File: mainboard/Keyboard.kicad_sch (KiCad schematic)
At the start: 111 parts, among them J10 Joystick, J11 Keyboard, J9 Cassette, Q3 TIS92, Q4 TIS92, Q5 TIS92, Q6 TIS92, Q7 TIS92, Q8 TIS92, Q9 TIS92, U21 RC4558, U36 TMS9901, U37 74LS156, U38 TIL119, U39 TIL119

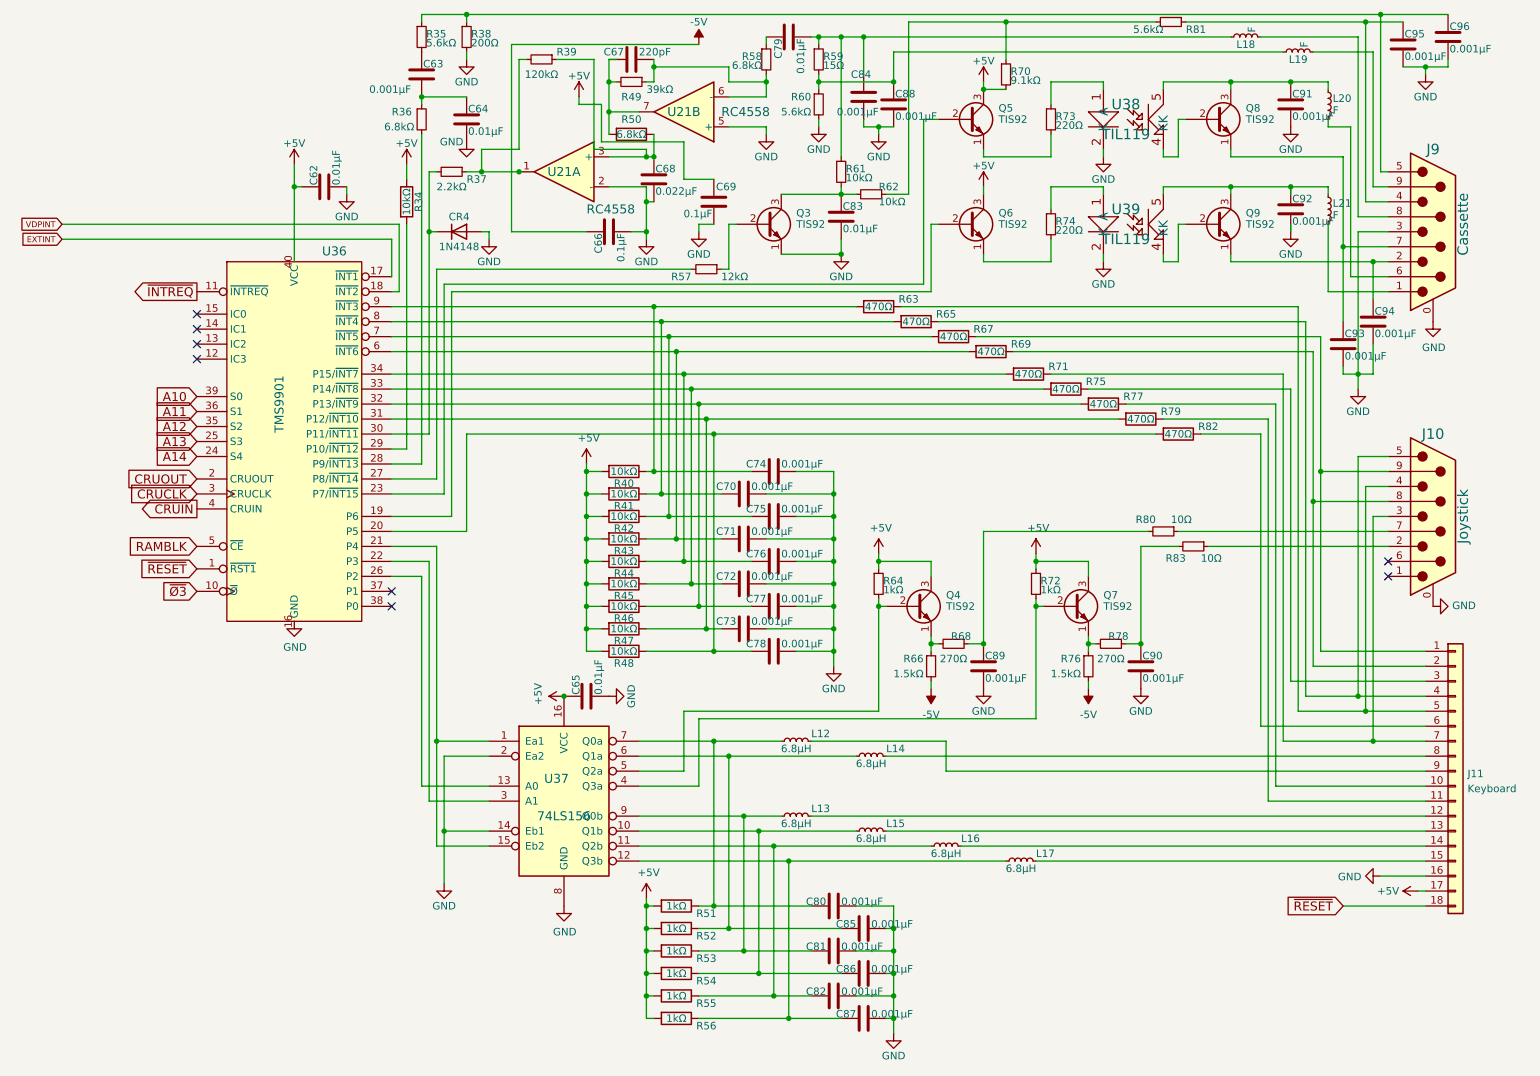
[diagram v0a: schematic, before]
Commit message: PCB rework
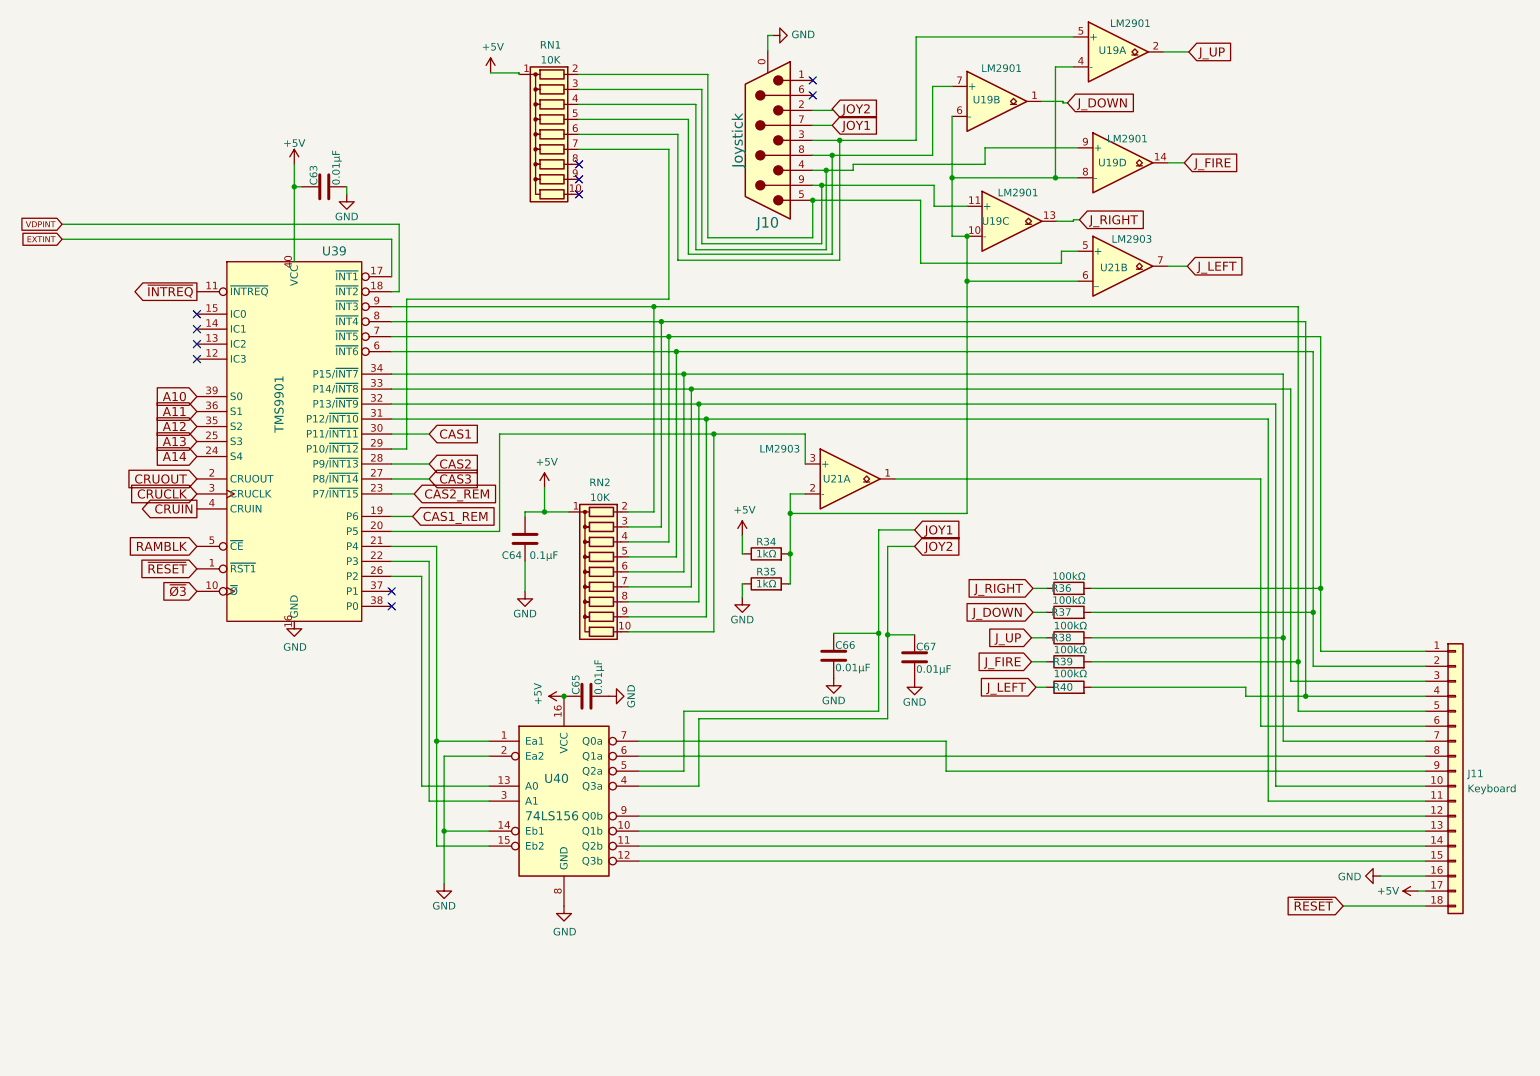
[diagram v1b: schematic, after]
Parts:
- removed C63, C70, C71, C72, C73, C75, C76, C77, C78, C80, C81, C82, C84, C85, C86, C87, C88, C91, C92, C93, C94, C95, C96: 0.001µF, Capacitor_THT:C_Rect_L7.0mm_W2.0mm_P5.00mm, symbol Device:C
- removed C64, C79, C83: 0.01µF, Capacitor_THT:C_Rect_L7.0mm_W2.0mm_P5.00mm, symbol Device:C
- removed C66, C69: 0.1µF, Capacitor_THT:C_Rect_L7.0mm_W2.0mm_P5.00mm, symbol Device:C
- removed C67: 220pF, Capacitor_THT:C_Rect_L7.0mm_W2.0mm_P5.00mm, symbol Device:C
- removed C68: 0.022µF, Capacitor_THT:C_Rect_L7.0mm_W2.0mm_P5.00mm, symbol Device:C
- removed CR4: 1N4148, Diode_THT:D_A-405_P7.62mm_Horizontal, symbol Device:D
- removed J9: Cassette, Connector_Dsub:DSUB-9_Female_Horizontal_P2.77x2.84mm_EdgePinOffset4.94mm_Housed_MountingHolesOffset7.48mm, symbol Connector:DB9_Male_MountingHoles
- removed L12, L13, L14, L15, L16, L17: 6.8µH, Resistor_THT:R_Axial_DIN0207_L6.3mm_D2.5mm_P7.62mm_Horizontal, symbol Device:L_Small
- removed L18, L19, L20, L21: F, Resistor_THT:R_Axial_DIN0207_L6.3mm_D2.5mm_P7.62mm_Horizontal, symbol Device:L_Small
- removed Q3, Q4, Q5, Q6, Q7, Q8, Q9: TIS92, Package_TO_SOT_THT:TO-92_HandSolder, symbol Device:Q_NPN_EBC
- removed R35, R60, R81: 5.6kΩ, Resistor_THT:R_Axial_DIN0207_L6.3mm_D2.5mm_P7.62mm_Horizontal, symbol Device:R_Small
- removed R36, R58: 6.8kΩ, Resistor_THT:R_Axial_DIN0207_L6.3mm_D2.5mm_P7.62mm_Horizontal, symbol Device:R_Small
- removed R37: 2.2kΩ, Resistor_THT:R_Axial_DIN0207_L6.3mm_D2.5mm_P7.62mm_Horizontal, symbol Device:R_Small
- removed R38: 200Ω, Resistor_THT:R_Axial_DIN0207_L6.3mm_D2.5mm_P7.62mm_Horizontal, symbol Device:R_Small
- removed R39: 120kΩ, Resistor_THT:R_Axial_DIN0207_L6.3mm_D2.5mm_P7.62mm_Horizontal, symbol Device:R_Small
- removed R41, R42, R43, R44, R45, R46, R47, R48: 10kΩ, Resistor_THT:R_Axial_DIN0207_L6.3mm_D2.5mm_P7.62mm_Horizontal, symbol Device:R
- removed R49: 39kΩ, Resistor_THT:R_Axial_DIN0207_L6.3mm_D2.5mm_P7.62mm_Horizontal, symbol Device:R_Small
- removed R50: 6.8kΩ, Resistor_THT:R_Axial_DIN0207_L6.3mm_D2.5mm_P7.62mm_Horizontal, symbol Device:R
- removed R51, R52, R53, R54, R55, R56: 1kΩ, Resistor_THT:R_Axial_DIN0207_L6.3mm_D2.5mm_P7.62mm_Horizontal, symbol Device:R
- removed R57: 12kΩ, Resistor_THT:R_Axial_DIN0207_L6.3mm_D2.5mm_P7.62mm_Horizontal, symbol Device:R_Small
- removed R59: 15Ω, Resistor_THT:R_Axial_DIN0207_L6.3mm_D2.5mm_P7.62mm_Horizontal, symbol Device:R_Small
- removed R61, R62: 10kΩ, Resistor_THT:R_Axial_DIN0207_L6.3mm_D2.5mm_P7.62mm_Horizontal, symbol Device:R_Small
- removed R63, R65, R67, R69, R71, R75, R77, R79, R82: 470Ω, Resistor_THT:R_Axial_DIN0207_L6.3mm_D2.5mm_P7.62mm_Horizontal, symbol Device:R
- removed R64, R72: 1kΩ, Resistor_THT:R_Axial_DIN0207_L6.3mm_D2.5mm_P7.62mm_Horizontal, symbol Device:R_Small
- removed R66, R76: 1.5kΩ, Resistor_THT:R_Axial_DIN0207_L6.3mm_D2.5mm_P7.62mm_Horizontal, symbol Device:R_Small
- removed R68, R78: 270Ω, Resistor_THT:R_Axial_DIN0207_L6.3mm_D2.5mm_P7.62mm_Horizontal, symbol Device:R_Small
- removed R70: 9.1kΩ, Resistor_THT:R_Axial_DIN0207_L6.3mm_D2.5mm_P7.62mm_Horizontal, symbol Device:R_Small
- removed R73, R74: 220Ω, Resistor_THT:R_Axial_DIN0207_L6.3mm_D2.5mm_P7.62mm_Horizontal, symbol Device:R_Small
- removed R80, R83: 10Ω, Resistor_THT:R_Axial_DIN0207_L6.3mm_D2.5mm_P7.62mm_Horizontal, symbol Device:R_Small
- removed U21: RC4558, Package_DIP:DIP-8_W7.62mm_Socket_LongPads, symbol Amplifier_Operational:RC4558
- removed U38, U39: TIL119, Package_DIP:DIP-6_W7.62mm_Socket_LongPads, symbol Werner_custom:TIL119
- added R34: 1kΩ, Resistor_THT:R_Axial_DIN0207_L6.3mm_D2.5mm_P7.62mm_Horizontal, symbol Device:R
- added R36, R37, R38, R39: 100kΩ, Resistor_THT:R_Axial_DIN0207_L6.3mm_D2.5mm_P7.62mm_Horizontal, symbol Device:R
- added RN1, RN2: 10K, Resistor_THT:R_Array_SIP10, symbol Device:R_Network09
- added U19: LM2901, Package_DIP:DIP-14_W7.62mm_Socket_LongPads, symbol Comparator:LM2901
- added U21: LM2903, Package_DIP:DIP-8_W7.62mm_Socket_LongPads, symbol Comparator:LM2903
- C64: renamed from C74; value 0.001µF -> 0.1µF
- C66: renamed from C89; value 0.001µF -> 0.01µF
- C67: renamed from C90; value 0.001µF -> 0.01µF
- R35: renamed from R34; value 10kΩ -> 1kΩ
- R40: value 10kΩ -> 100kΩ
- renumbered C62 to C63, U36 to U39, U37 to U40
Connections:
- net +5V: now also C64.2, R34.1, RN1.1 (common), RN2.1 (common); no longer R35.1, R40.2
- net GND: now also C64.1, R35.1; no longer C64.2
- net CAS1_REM: now reaches U39.19 (P6)
- net at U39.20 (P5): now also RN2.10 (R9), U21.3 (+)
- net CAS2_REM: now reaches U39.23 (P7/~{INT15})
- net CAS3: now reaches U39.27 (P8/~{INT14})
- net CAS2: now reaches U39.28 (P9/~{INT13})
- net at U39.29 (P10/~{INT12}): now also RN1.7 (R6); no longer R35.2
- net CAS1: now reaches U39.30 (P11/~{INT11})
- net at U39.31 (P12/~{INT10}): now also J11.11 (Pin_11), RN2.9 (R8)
- net at U39.32 (P13/~{INT9}): now also J11.10 (Pin_10), RN2.8 (R7)
- net at U39.33 (P14/~{INT8}): now also J11.3 (Pin_3), RN2.7 (R6)
- net at U39.34 (P15/~{INT7}): now also J11.7 (Pin_7), R38.2, RN2.6 (R5)
- net at U39.6 (~{INT6}): now also J11.2 (Pin_2), R37.2, RN2.5 (R4)
- net at U39.7 (~{INT5}): now also J11.1 (Pin_1), R36.2, RN2.4 (R3)
- net at U39.8 (~{INT4}): now also J11.4 (Pin_4), R40.2, RN2.3 (R2)
- net at U40.10 (Q1b): now also J11.13 (Pin_13)
- net at U40.11 (Q2b): now also J11.14 (Pin_14)
- net at U40.12 (Q3b): now also J11.15 (Pin_15)
- net JOY2: now reaches U40.4 (Q3a)
- net JOY2: now also C67.1, J10.2
- net JOY1: now reaches U40.5 (Q2a)
- net JOY1: now also C66.1, J10.7
- net at U40.6 (Q1a): now also J11.8 (Pin_8)
- net at U40.7 (Q0a): now also J11.9 (Pin_9)
- net at U40.9 (Q0b): now also J11.12 (Pin_12)
- net at J10.3: now also RN1.6 (R5), U19.5 (+); no longer J11.7 (Pin_7)
- net at J11.5 (Pin_5): now also U39.9 (~{INT3}), R39.2, RN2.2 (R1); no longer J10.4
- net at J10.5: now also RN1.2 (R1), U21.5 (+); no longer J11.4 (Pin_4)
- net at J10.8: now also RN1.5 (R4), U19.7 (+); no longer J11.2 (Pin_2)
- net at J10.9: now also RN1.3 (R2), U19.11 (+); no longer J11.1 (Pin_1)
- net at J11.6 (Pin_6): now also U21.1
- new net: R34.2, R35.2, U19.10 (-), U19.4 (-), U19.6 (-), U19.8 (-), U21.2 (-), U21.6 (_)
- new net: J10.4, RN1.4 (R3), U19.9 (+)
- new net J_DOWN: R37.1, U19.1
- new net J_FIRE: R39.1, U19.14
- new net J_LEFT: R40.1, U21.7
- new net J_RIGHT: R36.1, U19.13
- new net J_UP: R38.1, U19.2
- no-connect marks 8 -> 11
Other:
- moved on the sheet: C64, C66, C67, J10, R35
